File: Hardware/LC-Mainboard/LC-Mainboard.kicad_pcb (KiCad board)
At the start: 2 copper layers, 103 x 63 mm, 9 parts, among them J1 Raspberry_Pi, J2 Charge Controller, U1 MAX3232IDW

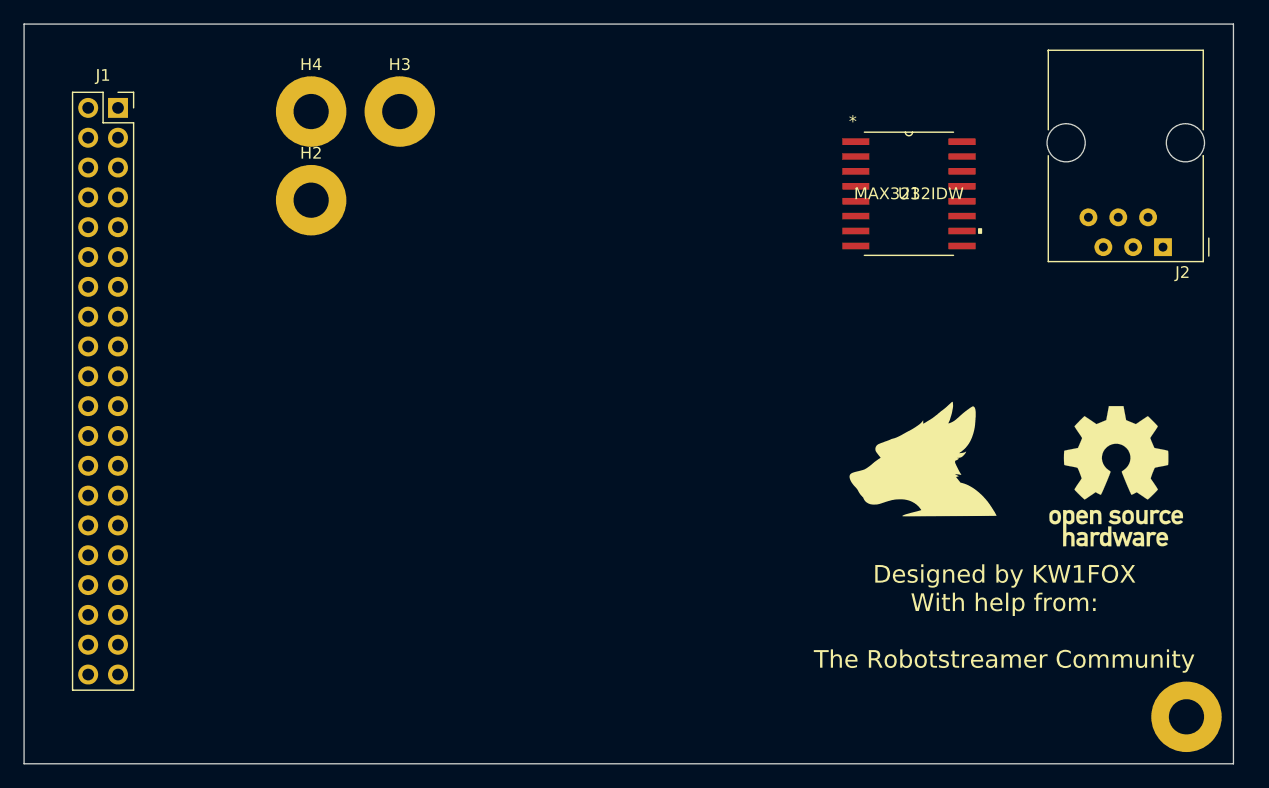
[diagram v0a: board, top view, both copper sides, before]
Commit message: Bump
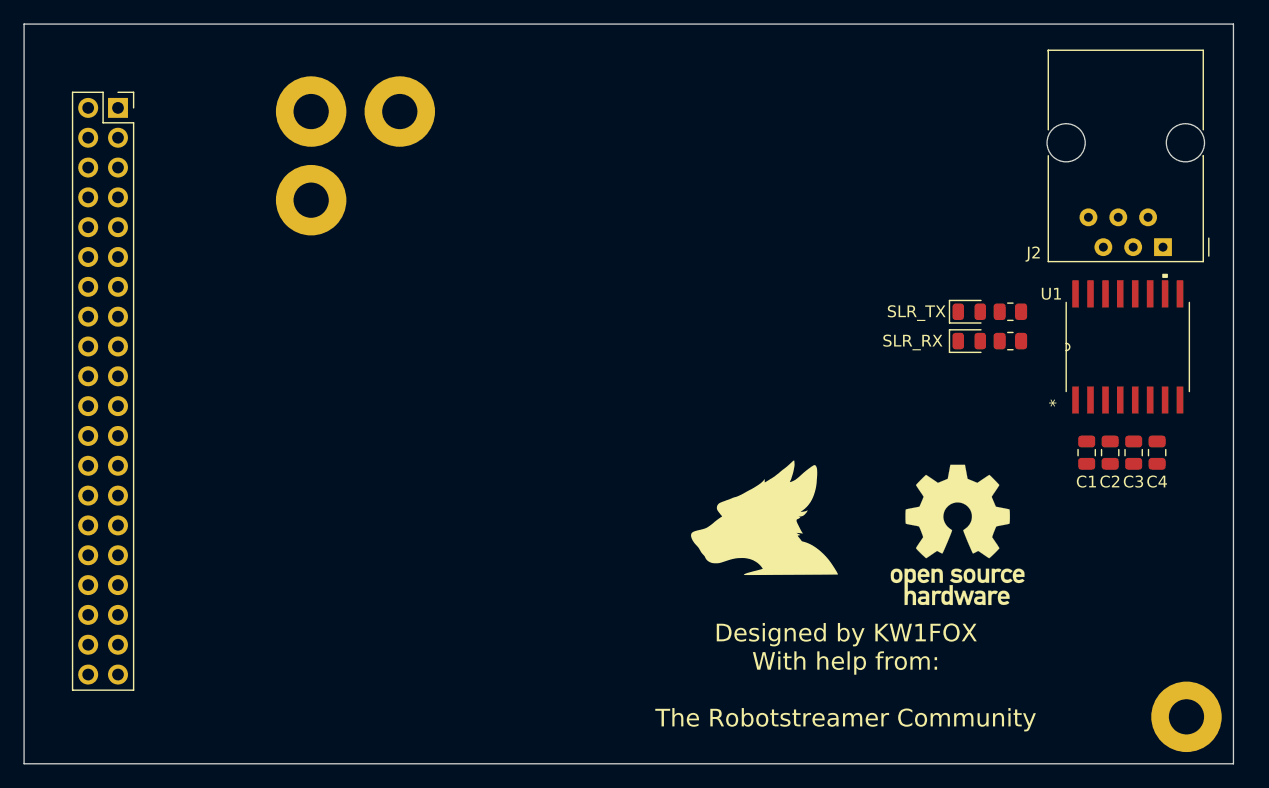
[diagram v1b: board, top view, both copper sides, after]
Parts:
- added C1: 0.1μf, Capacitor_SMD:C_0805_2012Metric, F.Cu at (191.5, 106.5)
- added C2: 0.1μf, Capacitor_SMD:C_0805_2012Metric, F.Cu at (193.5, 106.5)
- added C3: 0.1μf, Capacitor_SMD:C_0805_2012Metric, F.Cu at (195.5, 106.5)
- added C4: 0.1μf, Capacitor_SMD:C_0805_2012Metric, F.Cu at (197.5, 106.5)
- added D1: SLR_RX, LED_SMD:LED_0805_2012Metric, F.Cu at (181.5, 97.0)
- added D2: SLR_TX, LED_SMD:LED_0805_2012Metric, F.Cu at (181.5, 94.5)
- added R1: 100k, Resistor_SMD:R_0805_2012Metric, F.Cu at (185.0, 97.0)
- added R2: 100k, Resistor_SMD:R_0805_2012Metric, F.Cu at (185.0, 94.5)
- moved U1 22.8 mm to (195.0, 97.5), turned to 90 degrees
- moved G*** 14.4 mm to (164.0, 112.0)
- moved REF** 14.4 mm to (180.5, 113.5)
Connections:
- J1 pad 1: unconnected-(J1-Pad1) -> +3V3
- J1 pad 10: unconnected-(J1-Pad10) -> PI_RX
- J1 pad 14: unconnected-(J1-Pad14) -> GND
- J1 pad 17: unconnected-(J1-Pad17) -> +3V3
- J1 pad 2: unconnected-(J1-Pad2) -> +5V
- J1 pad 20: unconnected-(J1-Pad20) -> GND
- J1 pad 25: unconnected-(J1-Pad25) -> GND
- J1 pad 30: unconnected-(J1-Pad30) -> GND
- J1 pad 34: unconnected-(J1-Pad34) -> GND
- J1 pad 39: unconnected-(J1-Pad39) -> GND
- J1 pad 4: unconnected-(J1-Pad4) -> +5V
- J1 pad 6: unconnected-(J1-Pad6) -> GND
- J1 pad 8: unconnected-(J1-Pad8) -> PI_TX
- J1 pad 9: unconnected-(J1-Pad9) -> GND
- U1 pad 1: unconnected-(U1-Pad1) -> Net-(U1-Pad1)
- U1 pad 11: unconnected-(U1-Pad11) -> PI_TX
- U1 pad 12: unconnected-(U1-Pad12) -> PI_RX
- U1 pad 13: unconnected-(U1-Pad13) -> REN_TX
- U1 pad 14: unconnected-(U1-Pad14) -> REN_RX
- U1 pad 15: unconnected-(U1-Pad15) -> GND
- U1 pad 16: unconnected-(U1-Pad16) -> +3V3
- U1 pad 2: unconnected-(U1-Pad2) -> Net-(U1-Pad2)
- U1 pad 3: unconnected-(U1-Pad3) -> Net-(U1-Pad3)
- U1 pad 4: unconnected-(U1-Pad4) -> Net-(U1-Pad4)
- U1 pad 5: unconnected-(U1-Pad5) -> Net-(U1-Pad5)
- U1 pad 6: unconnected-(U1-Pad6) -> Net-(U1-Pad6)
